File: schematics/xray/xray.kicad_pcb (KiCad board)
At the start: 4 copper layers, 130 x 65 mm, 103 parts, among them J1 USB_A, J2 USB_B_Micro, J3 USB_C_Receptacle_USB2.0, J4 USBASP, M1 VibroMotor, 3V, 8x2.7mm, Q1 IRF7413ZPbF, Q10 IRLML0030, Q11 IRLML0030, Q2 IRF7424PBF, Q3 IRLML0030, Q4 IRF7424PBF, Q5 IRLML0030, Q6 BC857, Q7 BC847, Q8 IRLML0030, Q9 IRLML0030, SW1 EC11W****, T1 Transformer_1P_1S, U1 IP5328P, U2 ATmega328P-A, U3 SN74LVC2T45DCUR, U4 SN74LVC2T45DCUR, U5 SN74LVC2T45DCUR, U6 Display_1.18inch_st7535, Y1 HC-49SM, 8MHz

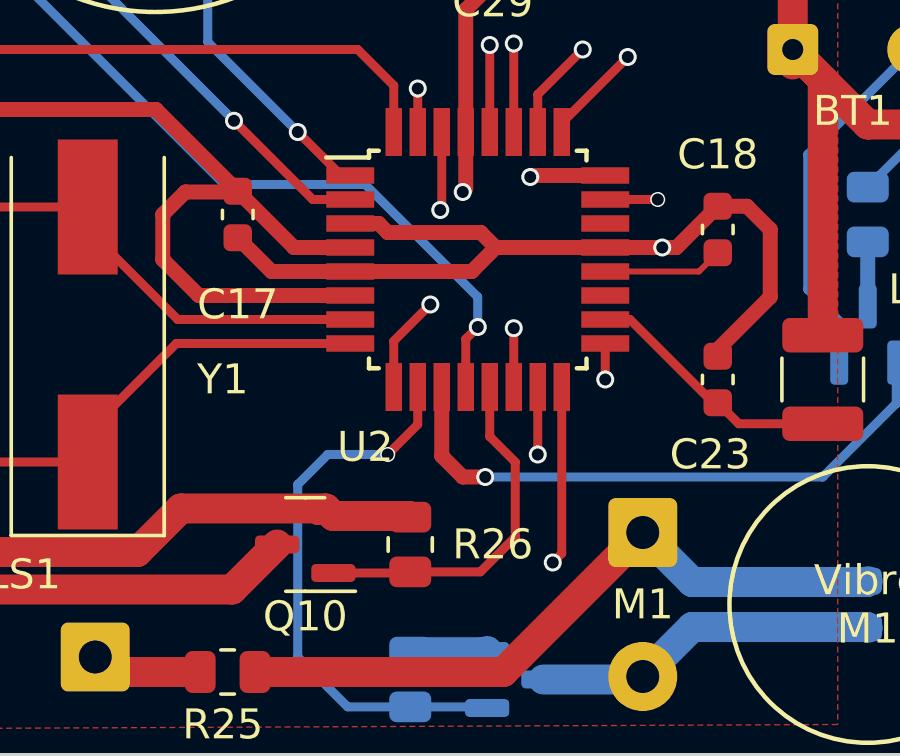
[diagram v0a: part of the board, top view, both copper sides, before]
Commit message: debugging...
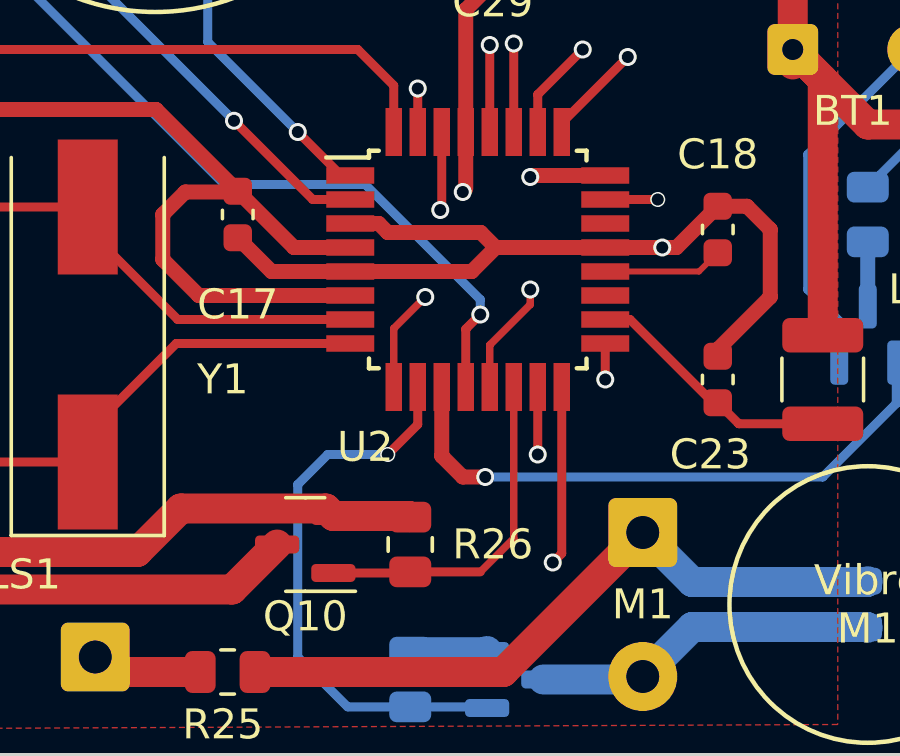
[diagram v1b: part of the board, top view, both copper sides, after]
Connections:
- U2 pad 13: SPEAKER -> USB_INT
- U2 pad 14: FLASHLIGHT -> SPEAKER
- U2 pad 9: USB_INT -> FLASHLIGHT
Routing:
- net FLASHLIGHT: track 61.8 -> 59.3 mm
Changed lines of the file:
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@@
       (net 37 "Net-(C31-Pad1)") (pinfunction "XTAL2/PB7") (pintype "bidirectional"))
     (pad "9" smd rect (at -2.8 4.25 90) (size 1.6 0.55) (layers "F.Cu" "F.Paste" "F.Mask")
-      (net 39 "USB_INT") (pinfunction "PD5") (pintype "bidirectional"))
+      (net 35 "FLASHLIGHT") (pinfunction "PD5") (pintype "bidirectional"))
     (pad "10" smd rect (at -2 4.25 90) (size 1.6 0.55) (layers "F.Cu" "F.Paste" "F.Mask")
       (net 38 "VIBRO") (pinfunction "PD6") (pintype "bidirectional"))
@@
       (net 45 "ENCODER_CLICK") (pinfunction "PB0") (pintype "bidirectional"))
     (pad "13" smd rect (at 0.4 4.25 90) (size 1.6 0.55) (layers "F.Cu" "F.Paste" "F.Mask")
-      (net 15 "SPEAKER") (pinfunction "PB1") (pintype "bidirectional"))
+      (net 39 "USB_INT") (pinfunction "PB1") (pintype "bidirectional"))
     (pad "14" smd rect (at 1.2 4.25 90) (size 1.6 0.55) (layers "F.Cu" "F.Paste" "F.Mask")
-      (net 35 "FLASHLIGHT") (pinfunction "PB2") (pintype "bidirectional"))
+      (net 15 "SPEAKER") (pinfunction "PB2") (pintype "bidirectional"))
     (pad "15" smd rect (at 2 4.25 90) (size 1.6 0.55) (layers "F.Cu" "F.Paste" "F.Mask")
       (net 59 "MOSI") (pinfunction "PB3") (pintype "bidirectional"))
@@
   (segment (start 78.01 101.54) (end 78.26 101.29) (width 1) (layer "F.Cu") (net 14))
   (segment (start 97.0475 101.04) (end 96.01 102.0775) (width 1) (layer "F.Cu") (net 14))
-  (segment (start 148.41 129.44) (end 149.26 130.29) (width 0.3) (layer "F.Cu") (net 15))
-  (segment (start 149.26 130.29) (end 149.26 132.79) (width 0.3) (layer "F.Cu") (net 15))
+  (segment (start 149.21 132.84) (end 149.21 127.79) (width 0.25) (layer "F.Cu") (net 15))
   (segment (start 148.0975 133.9525) (end 145.76 133.9525) (width 0.3) (layer "F.Cu") (net 15))
-  (segment (start 149.26 132.79) (end 148.0975 133.9525) (width 0.3) (layer "F.Cu") (net 15))
+  (segment (start 148.0975 133.9525) (end 149.21 132.84) (width 0.25) (layer "F.Cu") (net 15))
   (segment (start 145.7225 133.99) (end 145.76 133.9525) (width 0.3) (layer "F.Cu") (net 15))
   (segment (start 143.1975 133.99) (end 145.7225 133.99) (width 0.3) (layer "F.Cu") (net 15))
-  (segment (start 148.41 127.79) (end 148.41 129.44) (width 0.3) (layer "F.Cu") (net 15))
   (segment (start 175.055 109.065) (end 178.105 112.115) (width 1) (layer "F.Cu") (net 16))
   (segment (start 170.01 110.765) (end 170.035 110.74) (width 1) (layer "F.Cu") (net 16))
@@
   (segment (start 145.21 117.74) (end 145.21 119.29) (width 0.3) (layer "F.Cu") (net 34))
   (segment (start 103.51 112.1025) (end 101.01 114.6025) (width 0.5) (layer "F.Cu") (net 34))
-  (segment (start 149.21 125.8304) (end 149.21 127.79) (width 0.3) (layer "F.Cu") (net 35))
-  (via (at 149.21 125.8304) (size 0.6) (drill 0.4) (layers "F.Cu" "B.Cu") (net 35))
+  (segment (start 145.21 125.84) (end 145.21 127.79) (width 0.25) (layer "F.Cu") (net 35))
+  (segment (start 146.26 124.79) (end 145.21 125.84) (width 0.25) (layer "F.Cu") (net 35))
+  (via (at 146.26 124.79) (size 0.6) (drill 0.4) (layers "F.Cu" "B.Cu") (net 35))
   (via (at 110.96 120.09) (size 0.6) (drill 0.4) (layers "F.Cu" "B.Cu") (net 35))
-  (segment (start 124.01 124.04) (end 148.51 124.04) (width 0.3) (layer "In1.Cu") (net 35))
-  (segment (start 108.052894 128.79) (end 119.26 128.79) (width 0.3) (layer "In1.Cu") (net 35))
-  (segment (start 110.96 120.09) (end 107.01 124.04) (width 0.3) (layer "In1.Cu") (net 35))
-  (segment (start 107.01 124.04) (end 107.01 127.747106) (width 0.3) (layer "In1.Cu") (net 35))
-  (segment (start 119.26 128.79) (end 124.01 124.04) (width 0.3) (layer "In1.Cu") (net 35))
-  (segment (start 148.51 124.04) (end 149.21 124.74) (width 0.3) (layer "In1.Cu") (net 35))
-  (segment (start 107.01 127.747106) (end 108.052894 128.79) (width 0.3) (layer "In1.Cu") (net 35))
-  (segment (start 149.21 124.74) (end 149.21 125.8304) (width 0.3) (layer "In1.Cu") (net 35))
+  (segment (start 146.26 124.79) (end 145.51 124.04) (width 0.3) (layer "In1.Cu") (net 35))
+  (segment (start 124.01 124.04) (end 119.26 128.79) (width 0.3) (layer "In1.Cu") (net 35))
+  (segment (start 119.26 128.79) (end 108.052894 128.79) (width 0.3) (layer "In1.Cu") (net 35))
+  (segment (start 145.51 124.04) (end 124.01 124.04) (width 0.3) (layer "In1.Cu") (net 35))
+  (segment (start 108.052894 128.79) (end 107.01 127.747106) (width 0.3) (layer "In1.Cu") (net 35))
+  (segment (start 107.01 124.04) (end 110.96 120.09) (width 0.3) (layer "In1.Cu") (net 35))
+  (segment (start 107.01 127.747106) (end 107.01 124.04) (width 0.3) (layer "In1.Cu") (net 35))
   (segment (start 108.9475 120.09) (end 110.96 120.09) (width 0.3) (layer "B.Cu") (net 35))
   (segment (start 113.4725 120.09) (end 113.51 120.1275) (width 0.3) (layer "B.Cu") (net 35))
@@
   (segment (start 143.6725 138.4525) (end 142.26 137.04) (width 0.3) (layer "B.Cu") (net 38))
   (segment (start 142.01 131.04) (end 143.01 130.04) (width 0.3) (layer "B.Cu") (net 38))
+  (segment (start 149.76 125.04) (end 148.41 126.39) (width 0.25) (layer "F.Cu") (net 39))
+  (segment (start 148.41 126.39) (end 148.41 127.79) (width 0.25) (layer "F.Cu") (net 39))
+  (segment (start 149.76 124.54) (end 149.76 125.04) (width 0.25) (layer "F.Cu") (net 39))
   (segment (start 166.009999 101.79) (end 167.06 101.79) (width 0.2) (layer "F.Cu") (net 39))
   (segment (start 165.858175 101.638176) (end 166.009999 101.79) (width 0.2) (layer "F.Cu") (net 39))
-  (segment (start 145.21 126.259239) (end 145.21 127.79) (width 0.3) (layer "F.Cu") (net 39))
-  (segment (start 146.429239 125.04) (end 145.21 126.259239) (width 0.3) (layer "F.Cu") (net 39))
-  (via (at 146.429239 125.04) (size 0.6) (drill 0.4) (layers "F.Cu" "B.Cu") (net 39))
+  (via (at 149.76 124.54) (size 0.6) (drill 0.4) (layers "F.Cu" "B.Cu") (net 39))
   (via (at 165.858175 101.638176) (size 0.6) (drill 0.4) (layers "F.Cu" "B.Cu") (net 39))
+  (segment (start 152.16 122.14) (end 154.258529 122.14) (width 0.3) (layer "In2.Cu") (net 39))
+  (segment (start 149.76 124.54) (end 152.16 122.14) (width 0.3) (layer "In2.Cu") (net 39))
+  (segment (start 154.61 121.788529) (end 154.61 116.859239) (width 0.3) (layer "In2.Cu") (net 39))
   (segment (start 165.01 102.486351) (end 165.858175 101.638176) (width 0.3) (layer "In2.Cu") (net 39))
-  (segment (start 146.429239 125.04) (end 165.01 106.459239) (width 0.3) (layer "In2.Cu") (net 39))
+  (segment (start 154.61 116.859239) (end 165.01 106.459239) (width 0.3) (layer "In2.Cu") (net 39))
+  (segment (start 154.258529 122.14) (end 154.61 121.788529) (width 0.3) (layer "In2.Cu") (net 39))
   (segment (start 165.01 106.459239) (end 165.01 102.486351) (width 0.3) (layer "In2.Cu") (net 39))
   (segment (start 100.0975 120.04) (end 99.5475 120.59) (width 0.5) (layer "F.Cu") (net 40))
@@
   (segment (start 114.4 111.79) (end 116.985 111.79) (width 1) (layer "B.Cu") (net 44))
   (segment (start 113.15 110.54) (end 114.4 111.79) (width 1) (layer "B.Cu") (net 44))
-  (segment (start 148.01 125.79) (end 147.61 126.19) (width 0.3) (layer "F.Cu") (net 45))
-  (segment (start 147.61 126.19) (end 147.61 127.79) (width 0.3) (layer "F.Cu") (net 45))
-  (via (at 148.01 125.79) (size 0.6) (drill 0.4) (layers "F.Cu" "B.Cu") (net 45))
-  (segment (start 148.01 125.79) (end 148.01 124.79) (width 0.3) (layer "B.Cu") (net 45))
-  (segment (start 144.26 121.04) (end 139.564213 121.04) (width 0.3) (layer "B.Cu") (net 45))
+  (segment (start 148.094266 125.374266) (end 147.61 125.858532) (width 0.3) (layer "F.Cu") (net 45))
+  (segment (start 147.61 125.858532) (end 147.61 127.79) (width 0.3) (layer "F.Cu") (net 45))
+  (via (at 148.094266 125.374266) (size 0.6) (drill 0.4) (layers "F.Cu" "B.Cu") (net 45))
   (segment (start 124.51 108.815) (end 126.235 110.54) (width 1) (layer "B.Cu") (net 45))
-  (segment (start 148.01 124.79) (end 144.26 121.04) (width 0.3) (layer "B.Cu") (net 45))
-  (segment (start 126.235 110.54) (end 127.65 110.54) (width 1) (layer "B.Cu") (net 45))
   (segment (start 139.564213 121.04) (end 129.064213 110.54) (width 0.3) (layer "B.Cu") (net 45))
+  (segment (start 148.094266 125.374266) (end 148.094266 124.874266) (width 0.3) (layer "B.Cu") (net 45))
+  (segment (start 144.26 121.04) (end 139.564213 121.04) (width 0.3) (layer "B.Cu") (net 45))
+  (segment (start 126.235 110.54) (end 127.65 110.54) (width 1) (layer "B.Cu") (net 45))
   (segment (start 129.064213 110.54) (end 127.65 110.54) (width 0.3) (layer "B.Cu") (net 45))
+  (segment (start 148.094266 124.874266) (end 144.26 121.04) (width 0.3) (layer "B.Cu") (net 45))
   (segment (start 107.41 110.24) (end 107.51 110.34) (width 1) (layer "B.Cu") (net 46))
   (segment (start 58.51 110.24) (end 58.51 105.84) (width 1) (layer "B.Cu") (net 46))
